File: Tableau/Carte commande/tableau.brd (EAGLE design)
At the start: 109.2 x 90.3 mm, 42 parts, among them IC1 74LS47N, IC3 74LS47N, IC4 74LS47N, IC5 LM3914N, IC6 LM2576T

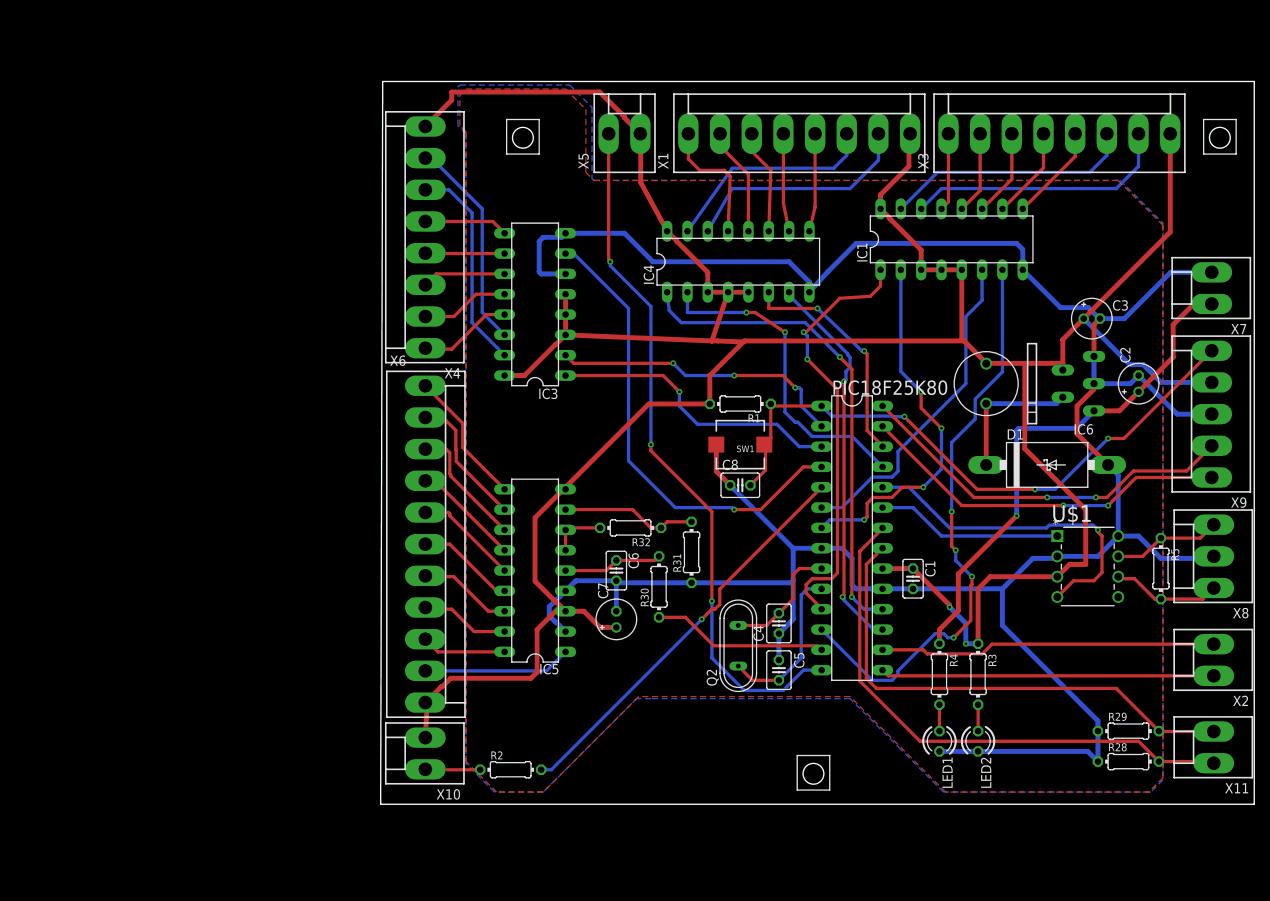
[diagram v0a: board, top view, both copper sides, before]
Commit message: no message
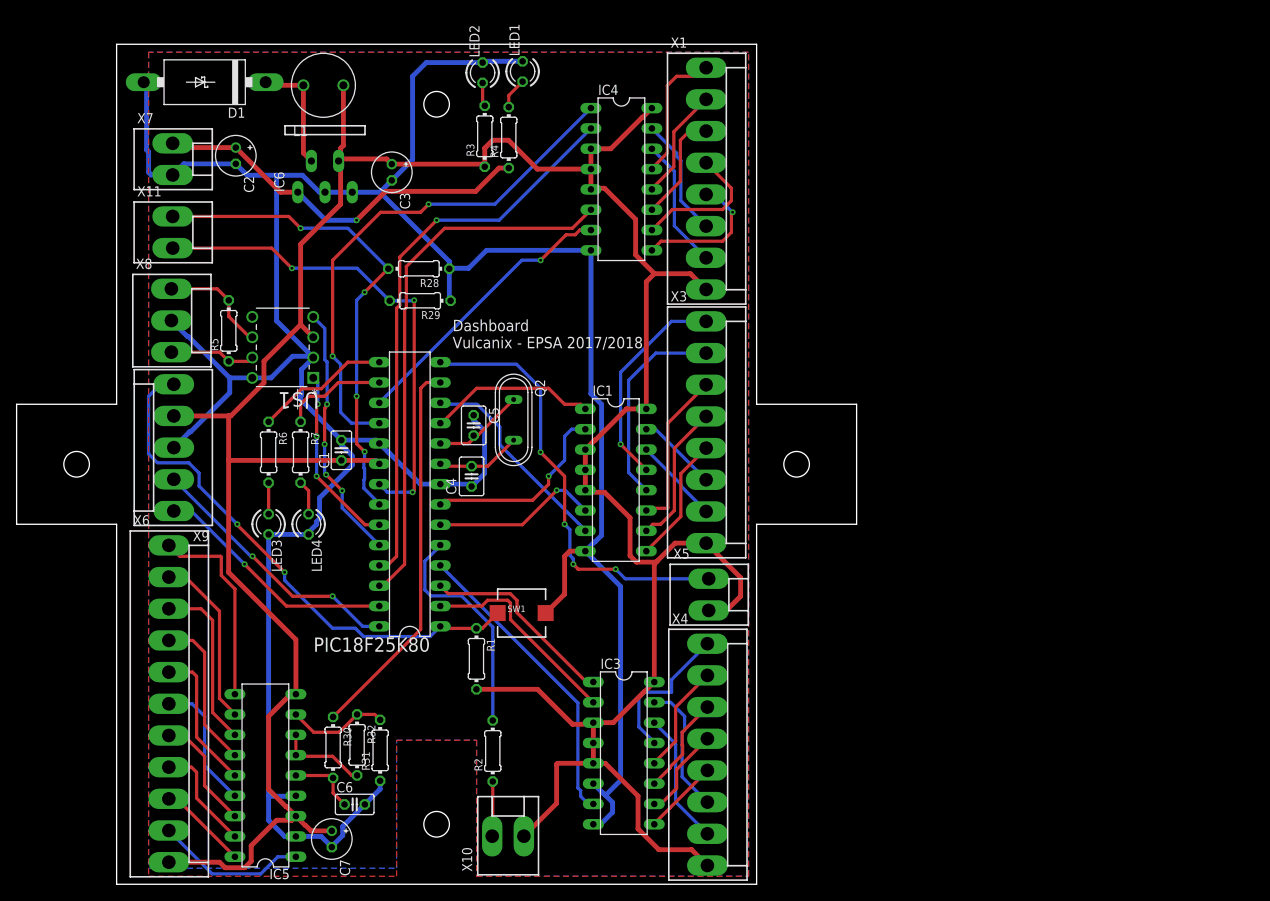
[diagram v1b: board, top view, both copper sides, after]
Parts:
- removed C8: (no value), rcl:C025-030X050
- removed X2: (no value), con-molex:KK-156-2
- added LED3, LED4: VERT, led:LED3MM
- added R6, R7: (no value), resistor:0204/7
- D1: value (none) -> 1N5822
- L1: value (none) -> 100uH
- R1: value (none) -> 10k
- moved X11 145.2 mm to (22.0, 71.5), turned to 270 degrees
- moved X8 133.6 mm to (21.9, 60.5), turned to 270 degrees
- moved X7 130.9 mm to (22.0, 80.6), turned to 270 degrees
- moved X9 129.8 mm to (22.1, 44.6)
- moved R5 120.3 mm to (29.0, 59.2), turned to 90 degrees
- moved C2 116.4 mm to (29.9, 81.1), turned to 270 degrees
- moved D1 115.7 mm to (26.0, 90.3), turned to 180 degrees
- moved U$1 113.8 mm to (32.0, 60.9), turned to 180 degrees
- moved R28 108.0 mm to (52.8, 66.9), turned to 180 degrees
- moved LED2 104.0 mm to (60.8, 91.4), turned to 90 degrees
- moved R29 103.6 mm to (52.9, 62.9), turned to 180 degrees
- moved LED1 98.6 mm to (65.8, 91.6), turned to 90 degrees
- moved IC6 93.5 mm to (41.0, 84.9), turned to 0 degrees
- moved R3 91.2 mm to (61.0, 83.5), turned to 90 degrees
- moved L1 90.9 mm to (40.9, 89.9), turned to 0 degrees
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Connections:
- removed net USB_D+: PIC18F25K80.16, X2.2
- removed net USB_D-: PIC18F25K80.15, X2.1
- new net LED_1: PIC18F25K80.16, R7.1
- new net LED_2: PIC18F25K80.15, R6.1
- new net N$38: LED3.A, R6.2
- new net N$39: LED4.A, R7.2
- net GND: now also LED3.K, LED4.K; no longer C8.1
- net MCLR: no longer C8.2
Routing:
- net D1EAU_0: track 72.6 -> 26.1 mm, vias 4 -> 0
- net GND: track 332.5 -> 379.0 mm
- net USB_D+: track 42.1 -> 0.00 mm
- net USB_D-: track 41.7 -> 0.00 mm
- net D0EAU_3: track 29.0 -> 67.6 mm, vias 2 -> 0
- net D1EAU_1: track 54.2 -> 21.0 mm, vias 2 -> 0
- net D2EAU: track 87.3 -> 55.3 mm, vias 3 -> 4
- net D0EAU_2: track 40.5 -> 70.7 mm, vias 2 -> 1
- net PWM_SHIFT: track 22.0 -> 48.4 mm
- net N$18: track 33.4 -> 10.8 mm
- net LED_HOMING: track 50.8 -> 28.5 mm, vias 1 -> 0
- net D1EAU_2: track 46.0 -> 24.4 mm, vias 4 -> 1
- net N$17: track 31.2 -> 10.1 mm
- net DRAP_0: track 58.6 -> 38.1 mm, vias 1 -> 0
- net D1EAU_3: track 41.0 -> 21.0 mm, vias 0 -> 1
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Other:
- board size 109.2 x 90.3 mm -> 105 x 105 mm
- board text added: "Dashboard Vulcanix - EPSA 2017/2018"
